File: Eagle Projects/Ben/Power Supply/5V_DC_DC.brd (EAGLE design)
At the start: 44 x 20 mm, 20 parts

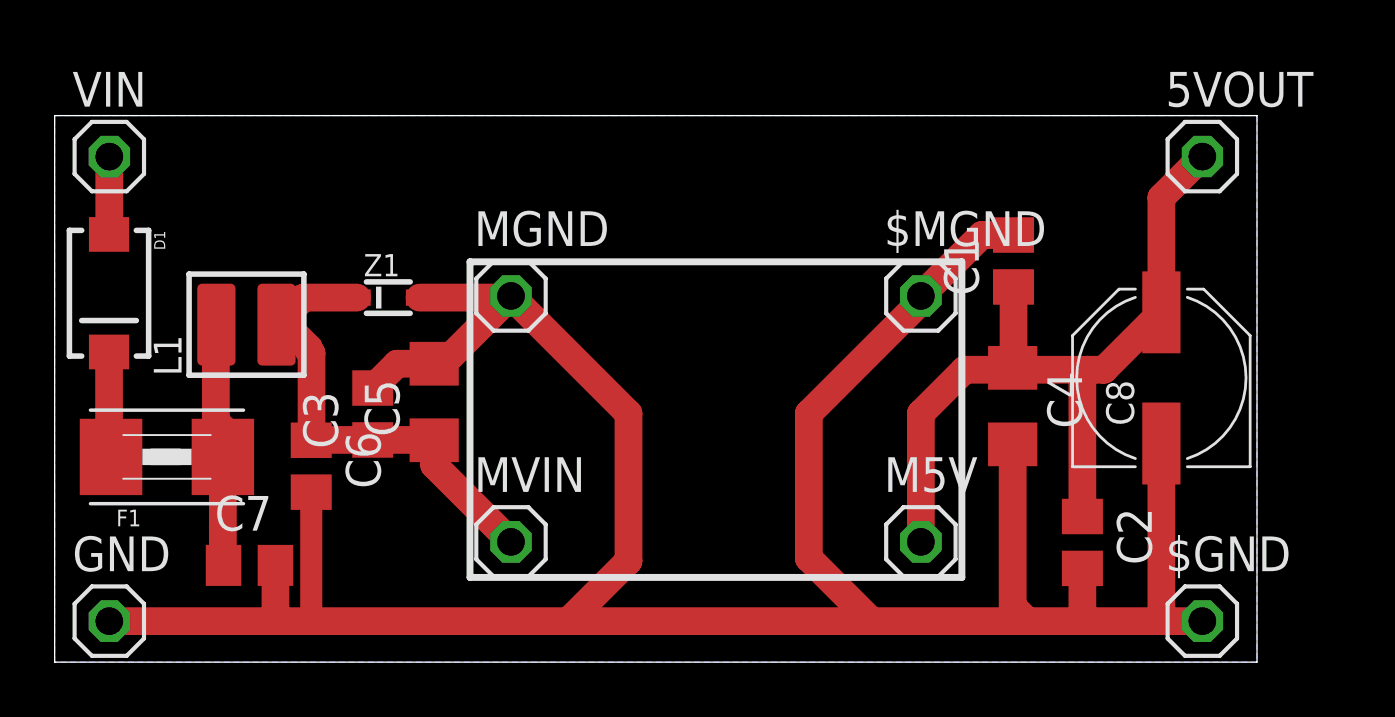
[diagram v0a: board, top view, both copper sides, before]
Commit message: Working on the things..
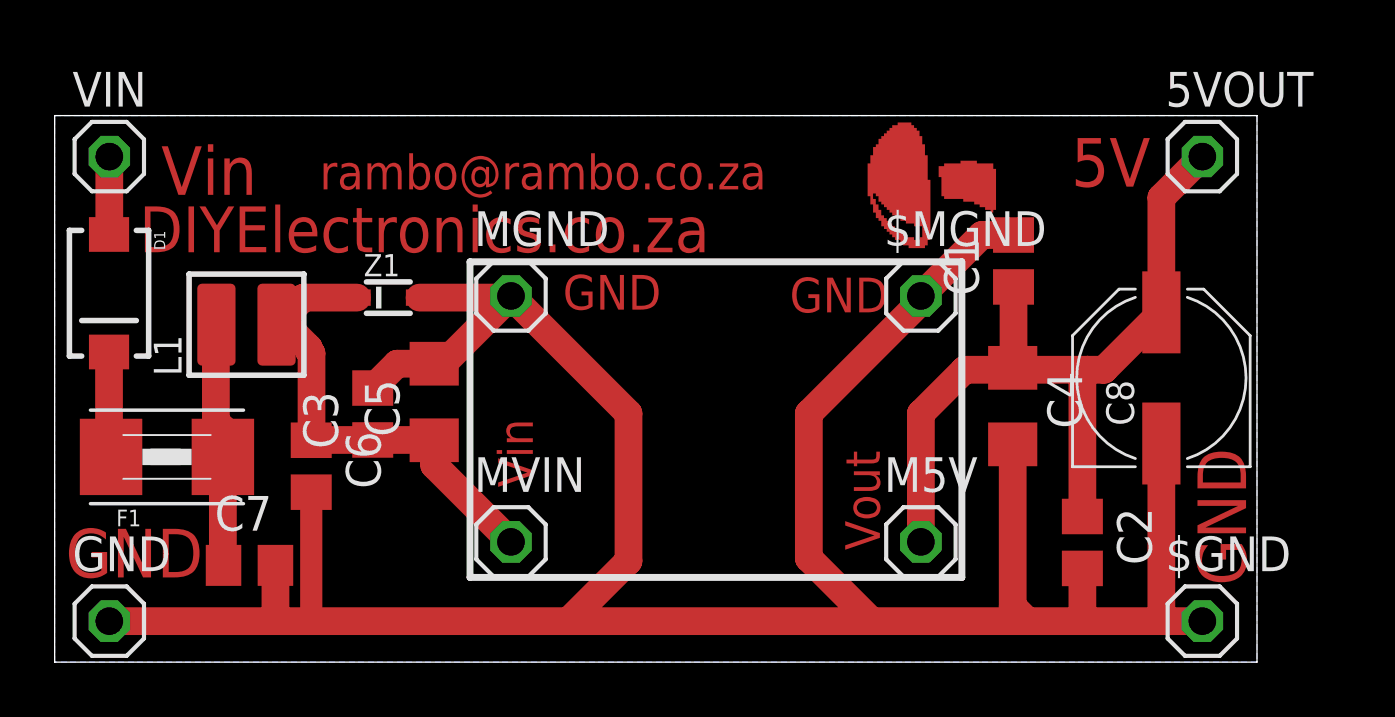
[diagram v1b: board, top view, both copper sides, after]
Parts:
- added U$1: SHROOM5MM, RobThePyro:SHROOM
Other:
- board text added: "5V"
- board text added: "DIYElectronics.co.za"
- board text added: "GND"
- board text added: "Vin"
- board text added: "Vout"
- board text added: "rambo@rambo.co.za"
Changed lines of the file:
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@@
 <layer number="56" name="wert" color="7" fill="1" visible="no" active="no"/>
 <layer number="57" name="tCAD" color="7" fill="1" visible="no" active="no"/>
+<layer number="59" name="tCarbon" color="7" fill="1" visible="no" active="no"/>
+<layer number="60" name="bCarbon" color="7" fill="1" visible="no" active="no"/>
 <layer number="90" name="Modules" color="5" fill="1" visible="no" active="no"/>
 <layer number="91" name="Nets" color="2" fill="1" visible="no" active="no"/>
@@
 <layer number="127" name="_tValues" color="7" fill="1" visible="yes" active="yes"/>
 <layer number="128" name="_bValues" color="7" fill="1" visible="yes" active="yes"/>
+<layer number="129" name="Mask" color="7" fill="1" visible="yes" active="yes"/>
 <layer number="131" name="tAdjust" color="7" fill="1" visible="no" active="yes"/>
 <layer number="132" name="bAdjust" color="7" fill="1" visible="no" active="yes"/>
@@
 <layer number="223" name="223bmp" color="24" fill="1" visible="no" active="no"/>
 <layer number="224" name="224bmp" color="25" fill="1" visible="no" active="no"/>
+<layer number="225" name="225bmp" color="7" fill="1" visible="yes" active="yes"/>
+<layer number="226" name="226bmp" color="7" fill="1" visible="yes" active="yes"/>
+<layer number="227" name="227bmp" color="7" fill="1" visible="yes" active="yes"/>
+<layer number="228" name="228bmp" color="7" fill="1" visible="yes" active="yes"/>
+<layer number="229" name="229bmp" color="7" fill="1" visible="yes" active="yes"/>
+<layer number="230" name="230bmp" color="7" fill="1" visible="yes" active="yes"/>
+<layer number="231" name="231bmp" color="7" fill="1" visible="yes" active="yes"/>
 <layer number="248" name="Housing" color="7" fill="1" visible="yes" active="yes"/>
 <layer number="249" name="Edge" color="7" fill="1" visible="yes" active="yes"/>
@@
 <layer number="251" name="SMDround" color="7" fill="1" visible="no" active="no"/>
 <layer number="254" name="cooling" color="7" fill="1" visible="yes" active="yes"/>
+<layer number="255" name="routoute" color="7" fill="1" visible="yes" active="yes"/>
 </layers>
 <board>
@@
 <wire x1="44" y1="20" x2="44" y2="0" width="0" layer="20"/>
 <wire x1="44" y1="0" x2="0" y2="0" width="0" layer="20"/>
+<text x="3.9" y="17.1" size="1.778" layer="1" ratio="20">Vin</text>
+<text x="37.2" y="17.4" size="1.778" layer="1" ratio="20">5V</text>
+<text x="0.4" y="3.1" size="1.778" layer="1" ratio="20">GND</text>
+<text x="43.6" y="2.8" size="1.778" layer="1" ratio="20" rot="R90">GND</text>
+<text x="3.1" y="15" size="1.6764" layer="1" ratio="15">DIYElectronics.co.za</text>
+<text x="9.7" y="17.3" size="1.27" layer="1" ratio="15">rambo@rambo.co.za</text>
+<text x="18.6" y="12.9" size="1.27" layer="1" ratio="15">GND</text>
+<text x="26.9" y="12.8" size="1.27" layer="1" ratio="15">GND</text>
+<text x="17.5" y="6.4" size="1.27" layer="1" ratio="15" rot="R90">Vin</text>
+<text x="30.2" y="4.1" size="1.27" layer="1" ratio="15" rot="R90">Vout</text>
 </plain>
 <attributes>
@@
 </element>
 <element name="C8" library="resistor" package="PANASONIC_D" value="" x="40.5" y="10.4" rot="R90"/>
+<element name="U$1" library="RobThePyro" package="SHROOM" value="SHROOM5MM" x="34.4" y="15.1" rot="R90"/>
 </elements>
 <signals>
